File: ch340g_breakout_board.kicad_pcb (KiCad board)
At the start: 2 copper layers, 31.8 x 20.3 mm, 9 parts, among them J1 Conn_01x08_Male, J2 Conn_01x08_Male, J3 XM7D-0512, U1 CH340G, Y1 12Mhz

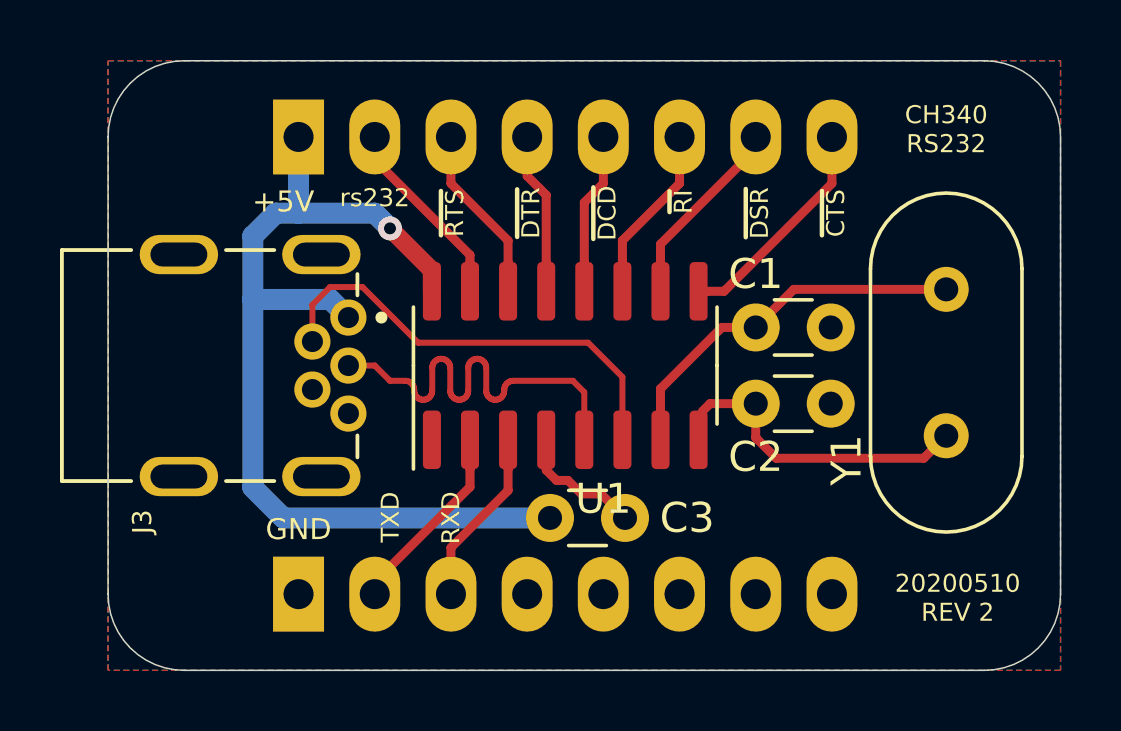
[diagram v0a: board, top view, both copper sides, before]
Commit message: Revision 2
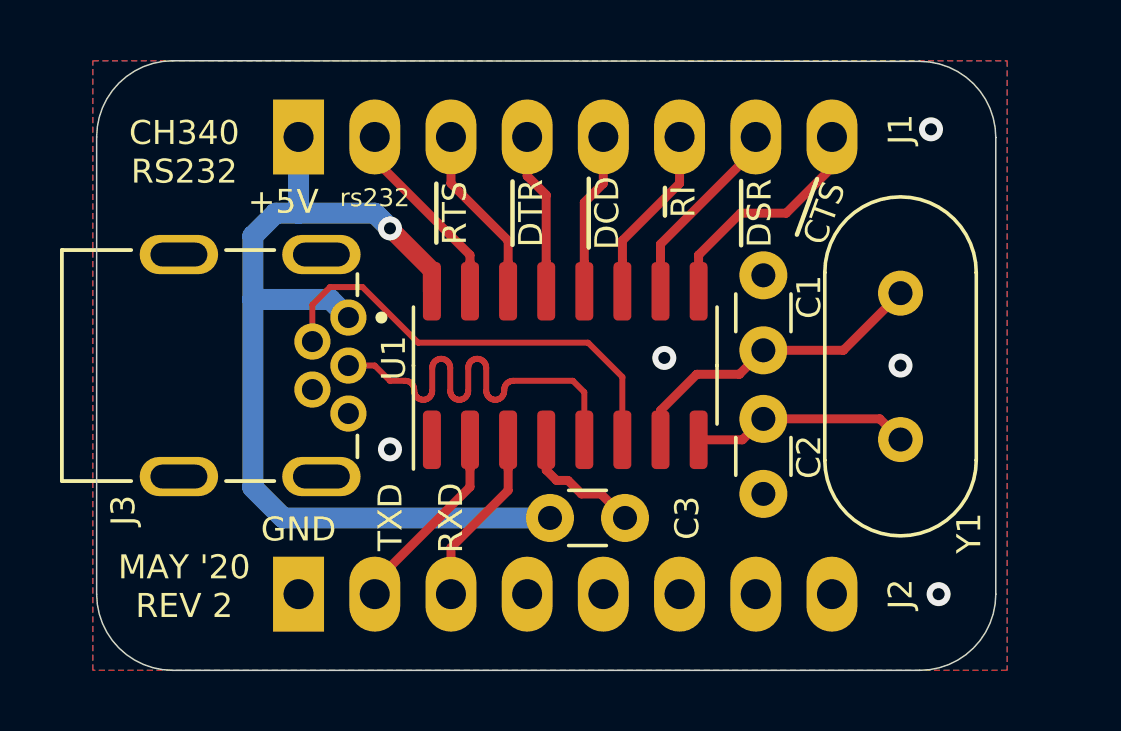
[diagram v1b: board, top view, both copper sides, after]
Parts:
- moved Y1 1.53 mm to (145.8, 99.2)
- moved REF** 1.14 mm to (134.5, 99.1)
- moved C1 0.80 mm to (141.2, 101.1), turned to 90 degrees
- moved C2 0.57 mm to (141.2, 103.4), turned to 270 degrees
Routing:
- net /XO: track 10.5 -> 7.31 mm
- net /XI: track 12.6 -> 10.6 mm
- net /GND: vias 0 -> 5
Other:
- board size 31.8 x 20.3 mm -> 30 x 20.3 mm
- board text added: "MAY '20 REV 2"
- board text removed: "20200510 REV 2"
